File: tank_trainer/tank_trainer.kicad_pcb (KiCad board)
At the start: 2 copper layers, 37.7 x 52.9 mm, 24 parts, among them U1 L7805, U2 ATMEGA328P-PU, Y1 Crystal

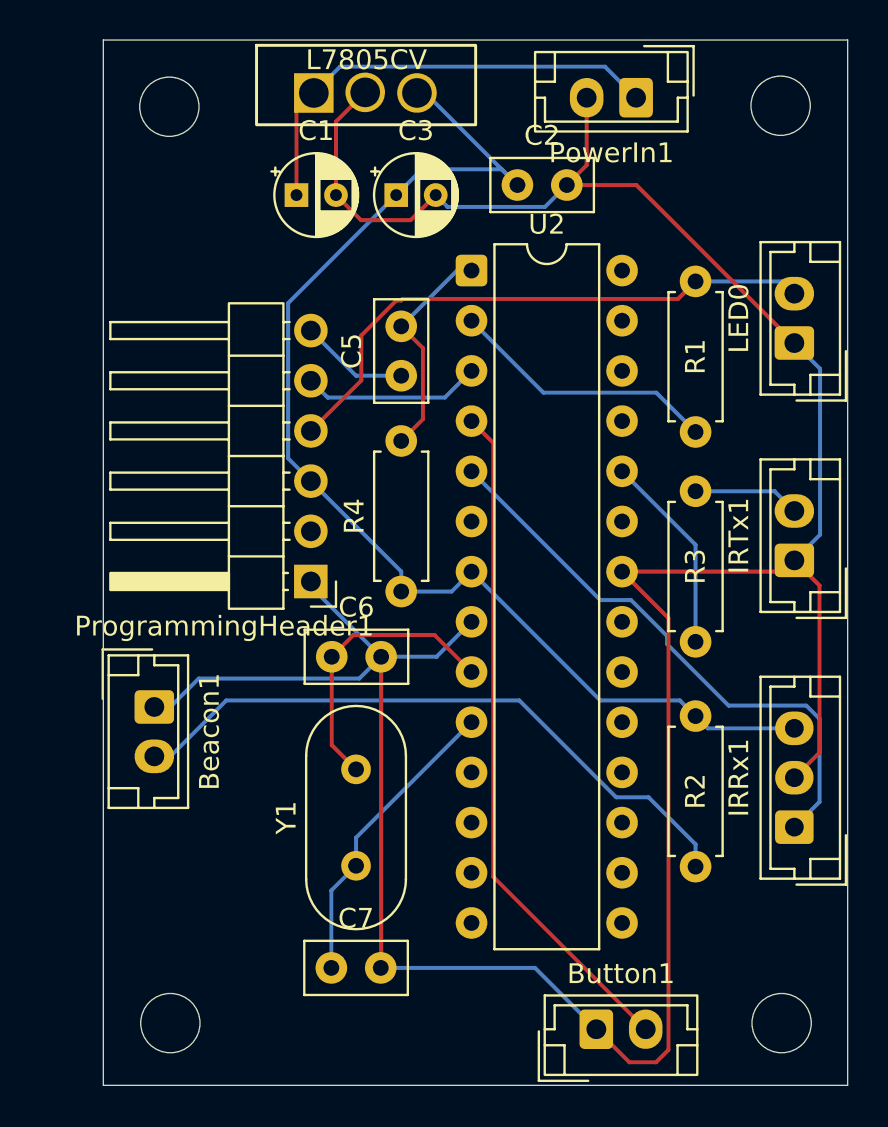
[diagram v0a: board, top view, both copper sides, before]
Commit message: Main Board v0.17 Tank Trainer v0.3
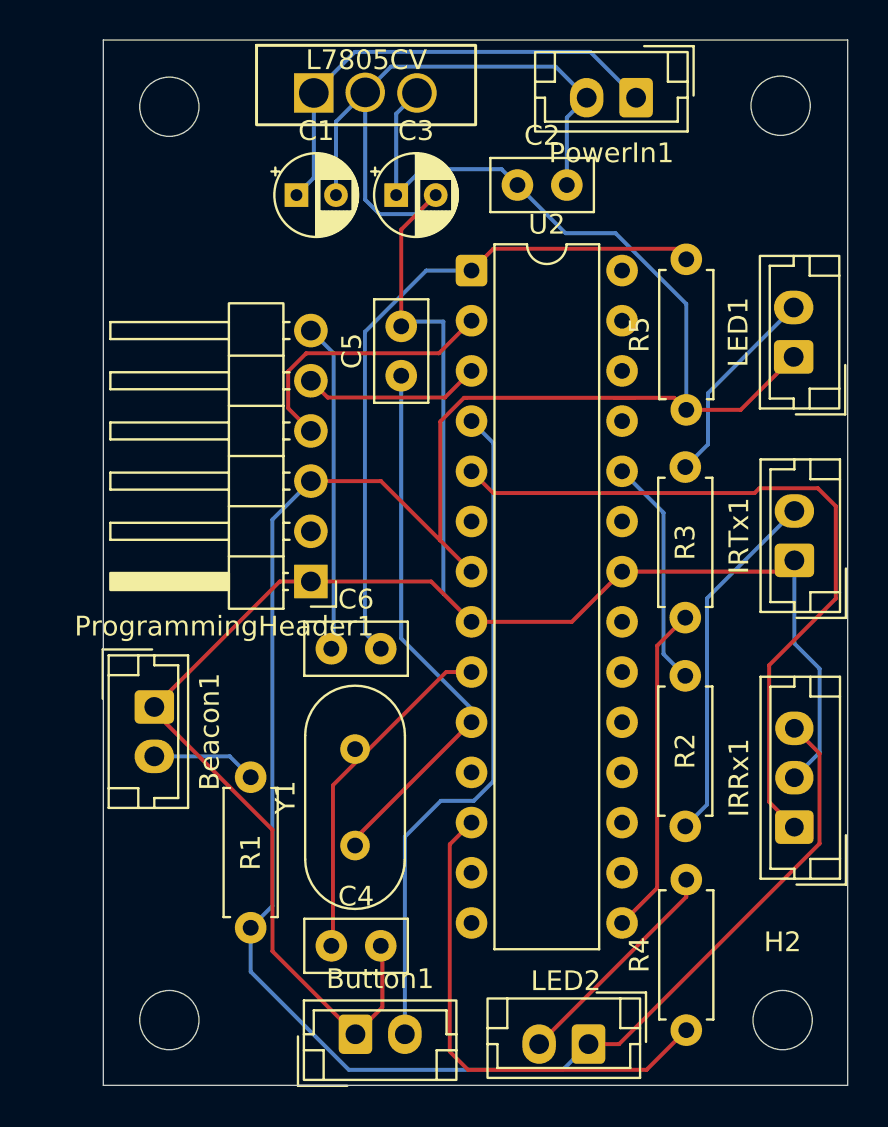
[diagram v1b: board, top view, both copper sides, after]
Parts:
- removed C7: 22pF, Capacitor_THT:C_Disc_D5.0mm_W2.5mm_P2.50mm
- removed H5: MountingHole, MountingHole:MountingHole_3mm
- removed LED0: Conn_01x02_Pin, Connector_JST:JST_EH_B2B-EH-A_1x02_P2.50mm_Vertical
- added C4: 22pF, Capacitor_THT:C_Disc_D5.0mm_W2.5mm_P2.50mm, F.Cu at (50.6, 118.0)
- added G***: LOGO, custom:Tank, B.Cu at (46.9, 102.7)
- added H2: MountingHole, MountingHole:MountingHole_3mm, F.Cu at (73.4, 121.8)
- added LED1: Conn_01x02_Pin, Connector_JST:JST_EH_B2B-EH-A_1x02_P2.50mm_Vertical, F.Cu at (74.0, 88.2)
- added LED2: Conn_01x02_Pin, Connector_JST:JST_EH_B2B-EH-A_1x02_P2.50mm_Vertical, F.Cu at (63.6, 123.0)
- added R5: R, Resistor_THT:R_Axial_DIN0207_L6.3mm_D2.5mm_P7.62mm_Horizontal, F.Cu at (68.5, 90.9)
- C5: value 100nF -> 22pF
- C6: value 22pF -> 100nF
- moved R1 33.7 mm to (46.5, 117.1)
- moved R4 26.5 mm to (68.5, 122.3)
- moved Button1 12.2 mm to (51.8, 122.5)
- moved R2 2.10 mm to (68.5, 104.3)
- moved R3 1.33 mm to (68.5, 101.4)
- moved Y1 1.03 mm to (51.8, 112.9)
- moved C6 0.41 mm to (50.6, 103.0)
- moved H4 0.16 mm to (42.4, 121.8)
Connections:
- C5 pad 1: Net-(ProgrammingHeader1-Pin_6) -> Net-(U2-(PCINT7/XTAL2/TOSC2)PB7)
- C5 pad 2: Net-(U2-(PCINT14/~{RESET})PC6) -> GND
- C6 pad 1: Net-(U2-(PCINT6/XTAL1/TOSC1)PB6) -> Net-(ProgrammingHeader1-Pin_6)
- C6 pad 2: GND -> Net-(U2-(PCINT14/~{RESET})PC6)
- R1 pad 1: Net-(U2-(PCINT16/RXD)PD0) -> 4.5V
- R1 pad 2: Rx -> Net-(Beacon1-Pin_2)
- R2 pad 1: 4.5V -> Net-(U2-(PCINT9/ADC1)PC1)
- R2 pad 2: Net-(Beacon1-Pin_2) -> Net-(IRTx1-Pin_2)
- R3 pad 1: Net-(U2-(PCINT9/ADC1)PC1) -> Net-(U2-(PCINT1/OC1A)PB1)
- R3 pad 2: Net-(IRTx1-Pin_2) -> Net-(LED1-Pin_2)
- R4 pad 1: 4.5V -> Net-(U2-(PCINT22/OC0A/AIN0)PD6)
- R4 pad 2: Net-(U2-(PCINT14/~{RESET})PC6) -> Net-(LED2-Pin_2)
- U2 pad 12: unconnected-(U2-(PCINT22/OC0A/AIN0)PD6-Pad12) -> Net-(U2-(PCINT22/OC0A/AIN0)PD6)
- U2 pad 15: unconnected-(U2-(PCINT1/OC1A)PB1-Pad15) -> Net-(U2-(PCINT1/OC1A)PB1)
- U2 pad 2: Net-(U2-(PCINT16/RXD)PD0) -> Rx
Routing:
- net 4.5V: track 62.3 -> 134.7 mm
- net Net-(Beacon1-Pin_2): track 32.6 -> 5.31 mm
- net Net-(U2-(PCINT22/OC0A/AIN0)PD6): track 0.00 -> 25.6 mm
- net Net-(U2-(PCINT14/~{RESET})PC6): track 11.4 -> 34.6 mm
- net GND: track 152.8 -> 132.9 mm
- net Net-(U2-(PCINT1/OC1A)PB1): track 0.00 -> 16.8 mm
- net Rx: track 29.2 -> 13.8 mm
- net Net-(U2-(PCINT16/RXD)PD0): track 13.7 -> 0.00 mm
- net Net-(IRTx1-Pin_2): track 5.41 -> 18.3 mm
- net Net-(U2-(PCINT7/XTAL2/TOSC2)PB7): track 15.4 -> 28.2 mm
- net Net-(LED2-Pin_2): track 0.00 -> 11.4 mm
- net Net-(ProgrammingHeader1-Pin_6): track 5.52 -> 16.6 mm
- net Net-(LED1-Pin_2): track 0.00 -> 10.3 mm
- net Net-(IRRx1-Pin_1): track 29.0 -> 37.5 mm
- net Net-(U2-(PCINT6/XTAL1/TOSC1)PB6): track 14.5 -> 17.8 mm
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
